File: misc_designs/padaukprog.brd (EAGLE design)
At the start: 100 x 100 mm, 144 parts, among them IC1 LM358D, J1 JUMPER_SOLDER_1X2, J2 JUMPER_SOLDER_1X2, J3 JST-PH 2mm, M1 XT1861B, M2 XT1861B, P1 B3B-PH-K, P2 B3B-PH-K, Q1 BSS84, Q2 8MHz, Q3 BSS84, Q4 BSS123, U1 MIC550X

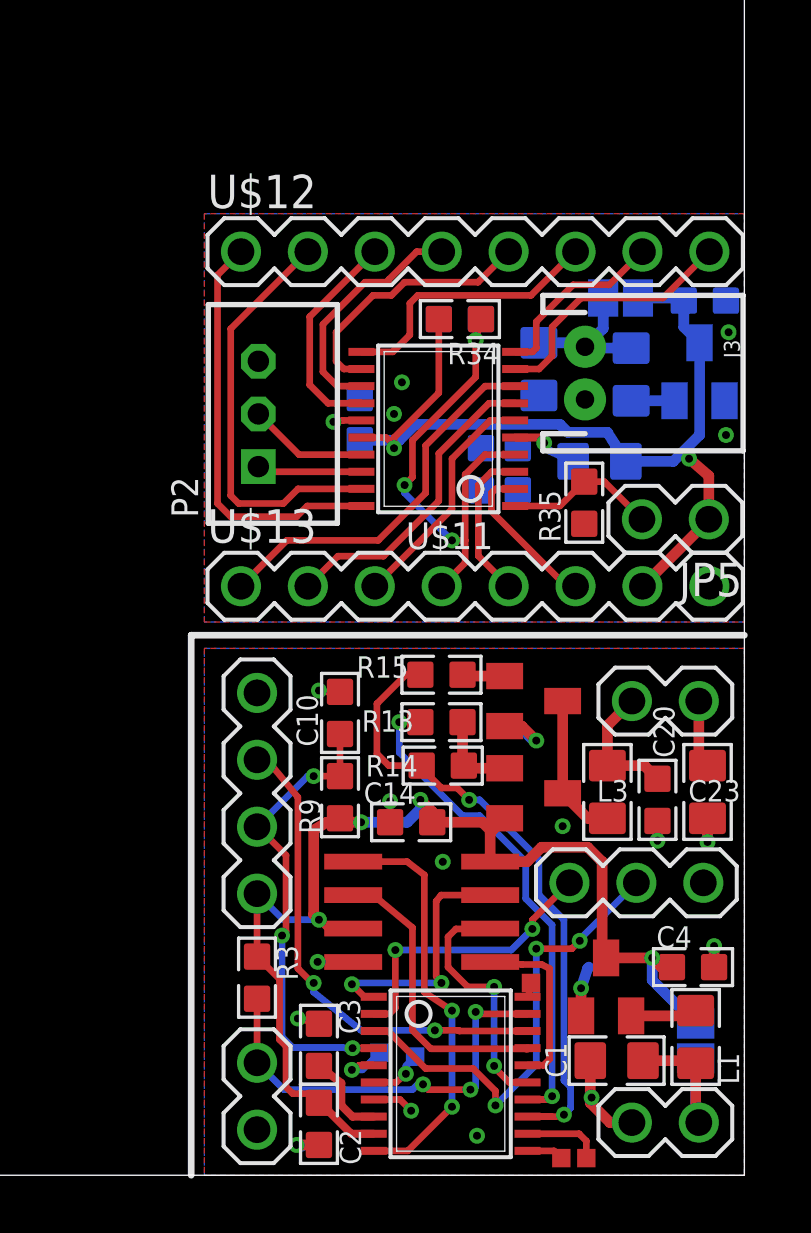
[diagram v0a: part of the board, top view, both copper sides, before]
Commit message: Cleanup
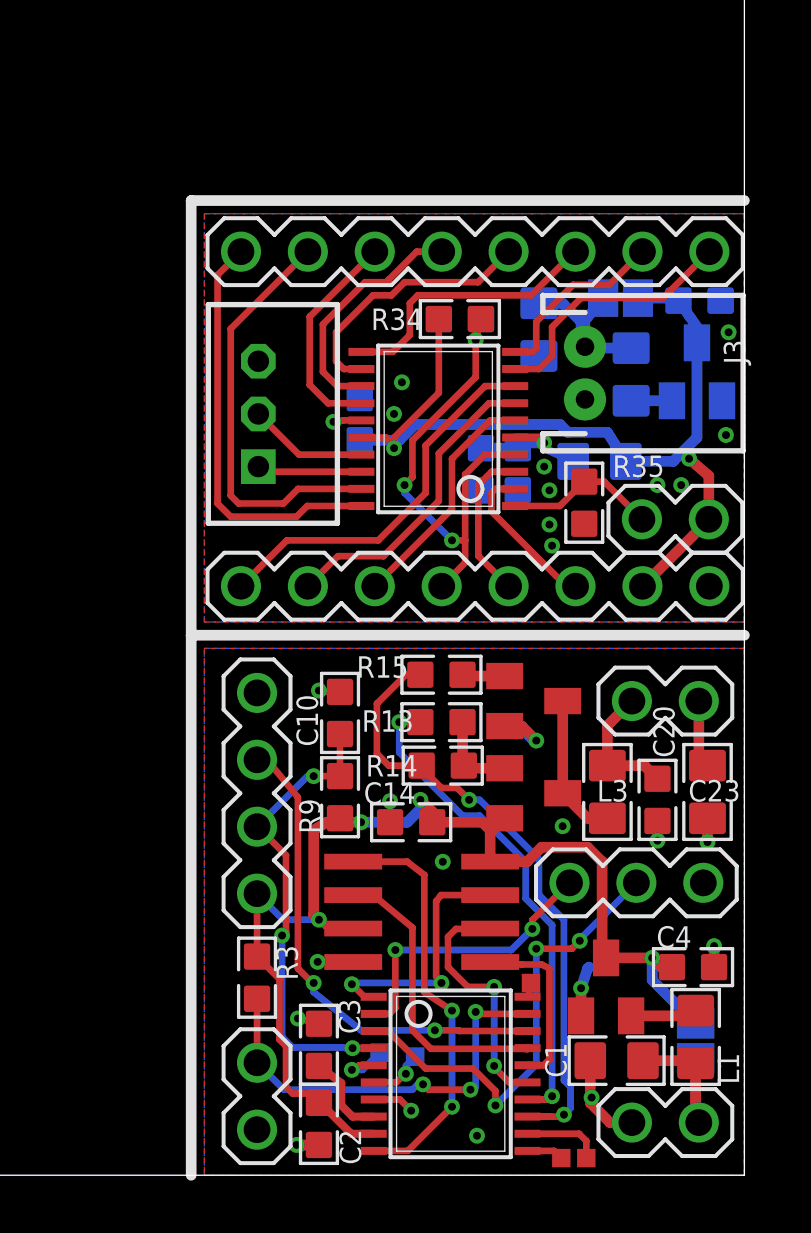
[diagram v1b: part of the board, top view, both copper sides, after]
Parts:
- moved C32 1.50 mm to (92.2, 32.1)
- moved C33 0.20 mm to (98.3, 33.2)
- moved M2 0.10 mm to (98.2, 30.5)
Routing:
- net +3V3: track 270.7 -> 282.4 mm
- net GND: track 34.0 -> 44.6 mm, vias 141 -> 147
- net N$10: track 2.71 -> 5.19 mm
- net N$13: track 5.72 -> 6.77 mm
